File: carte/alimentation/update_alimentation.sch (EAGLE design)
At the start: 34 parts, among them IC1 LM2596T, IC2 LM2596T, K1 RP811005, T1 2N2222, X10 22-23-2021, X11 22-23-2021, X9 22-23-2021

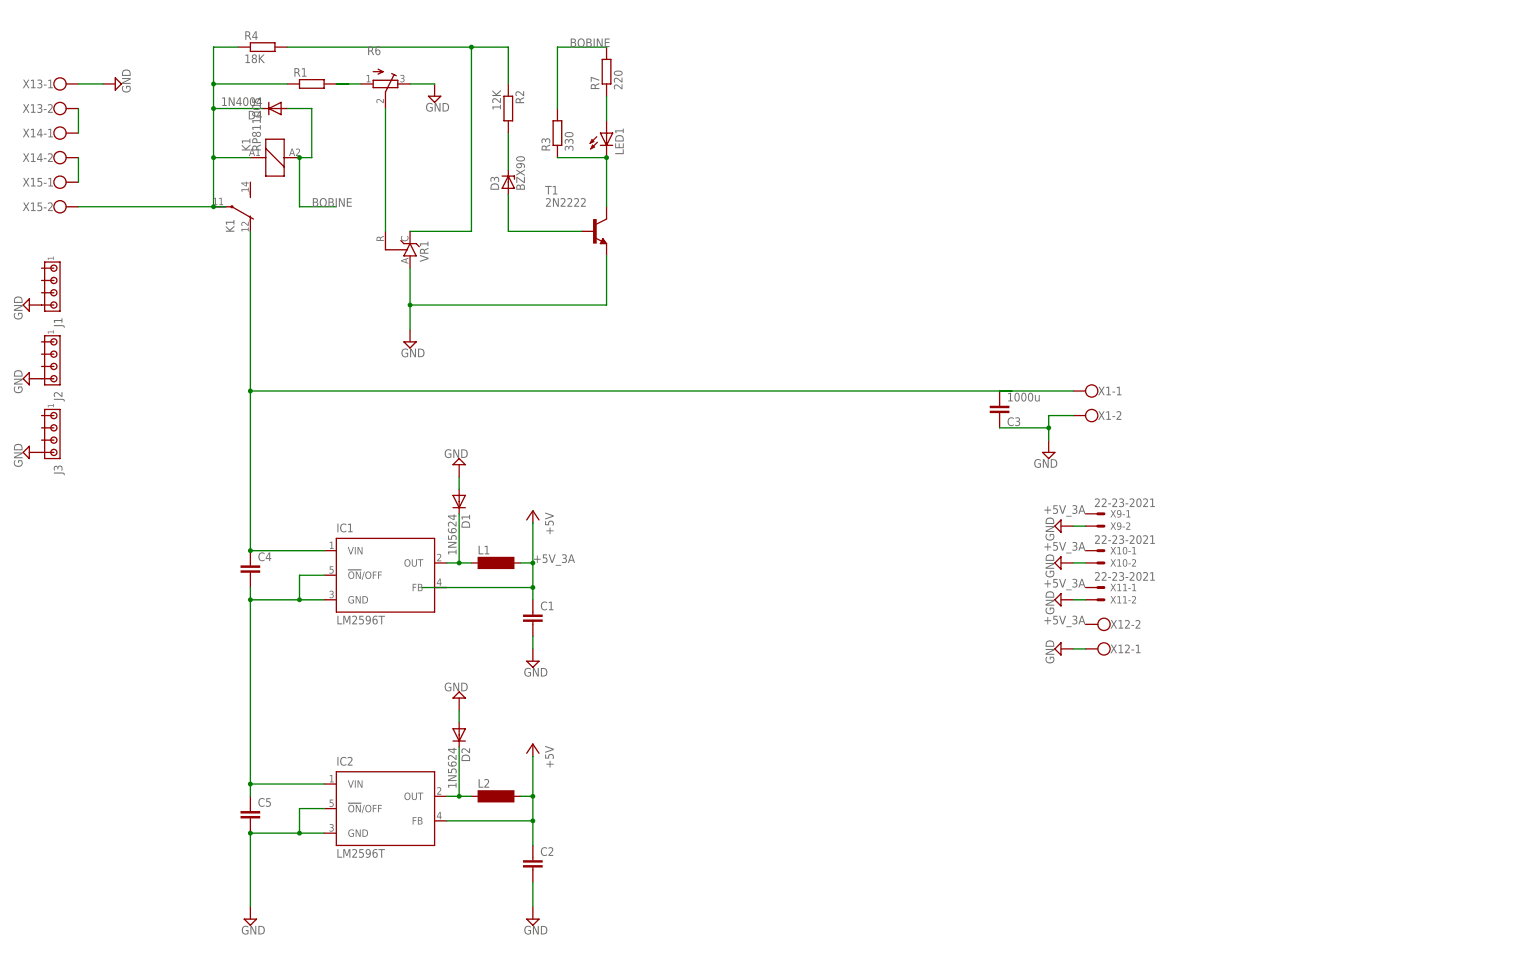
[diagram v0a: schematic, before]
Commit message: MAJ layout eagle
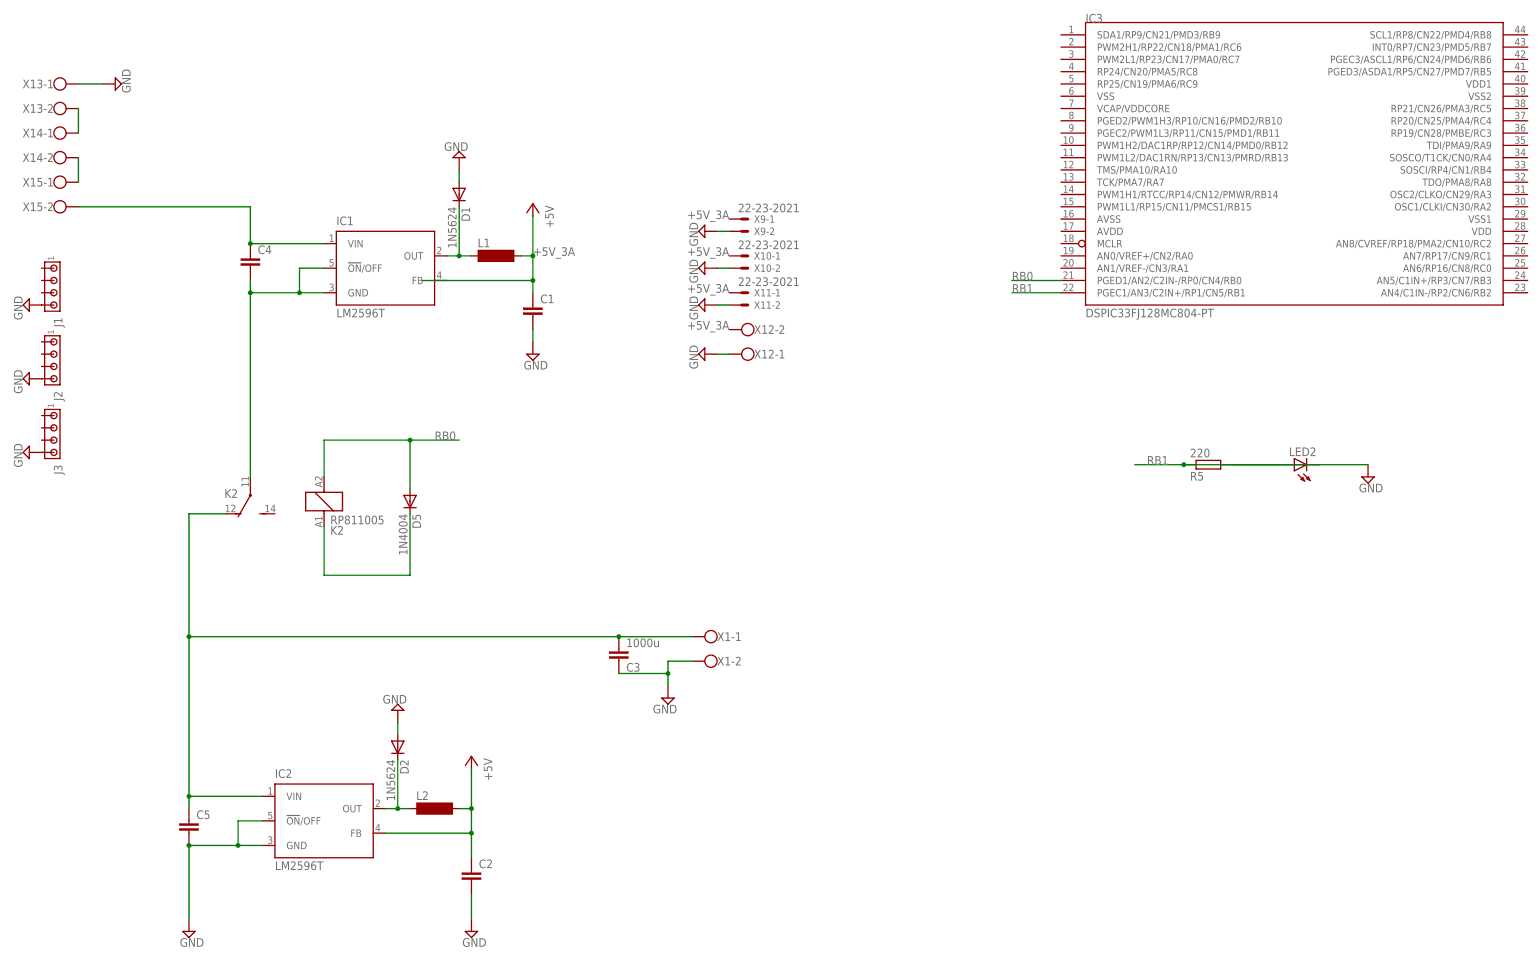
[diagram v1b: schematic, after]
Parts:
- removed D3: BZX90, diode:BZX90
- removed D4: 1N4004, diode:1N4004
- removed K1: RP811005, relay:RP811005
- removed LED1: (no value), eagle-ltspice:LED_E
- removed R1: (no value), resistor:R-EU_R0805
- removed R2: 12K, resistor:R-EU_R0805
- removed R3: 330, resistor:R-EU_R0805
- removed R4: 18K, resistor:R-EU_R0805
- removed R6: (no value), pot:TRIM_EU-3223G
- removed R7: 220, resistor:R-EU_R0805
- removed T1: 2N2222, transistor:2N2222
- removed VR1: (no value), v-reg:TL431CLP
- added D5: 1N4004, diode:1N4004
- added IC3: DSPIC33FJ128MC804-PT, microchip-dspic33fjxxmc:DSPIC33FJ128MC804-PT
- added K2: RP811005, relay:RP811005
- added LED2: (no value), eagle-ltspice:LED_E
- added R5: 220, resistor:R-EU_R0805
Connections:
- removed net BOBINE: D4.A, K11.2, R3.2, R7.2
- removed net N$10: D3.A, T1.B
- removed net N$14: LED1.A, R7.1
- removed net N$15: R6.S, VR1.R
- removed net N$2: D4.C, K11.1, K12.P, R1.1, R4.1, X15-2.KL
- removed net N$21: LED1.C, R3.1, T1.C
- removed net N$22: R2.1, R4.2, VR1.C
- removed net N$5: R1.2, R6.A
- removed net N$8: D3.C, R2.2
- new net N$16: D5.C, K21.1
- new net N$7: LED2.A, R5.2
- new net RB0: D5.A, IC3.PGED1/AN2/C2IN-/RP0/CN4/RB0, K21.2
- new net RB1: IC3.PGEC1/AN3/C2IN+/RP1/CN5/RB1, LED2.C, R5.1
- net GND: no longer R6.E, T1.E, VR1.A
- net N$11: now also X15-2.KL; no longer K12.O
- net N$13: now also C5.1, IC2.VIN, K22.O
- net N$6: now also K22.P; no longer C5.1, IC2.VIN
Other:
- moved on the sheet: C1, C2, C3, C4, C5, D1, D2, IC1, IC2, L1, L2, X1-1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
